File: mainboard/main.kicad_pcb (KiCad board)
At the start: 2 copper layers, 53.3 x 71.1 mm, 56 parts, among them J1 USB_OTG, J2 HIB, J3 JTAG Port, J4 C Port, J5 A Port, J6 E Port, J7 D Port, J8 B Port, J9 F Port, SW1 SW_Push, SW2 SW_Push, SW3 SW_Push, U1 LM1117-3.3, U2 TM4C123GH6PM, Y1 Crystal_GND24_Small, Y2 Crystal-32.768KHz

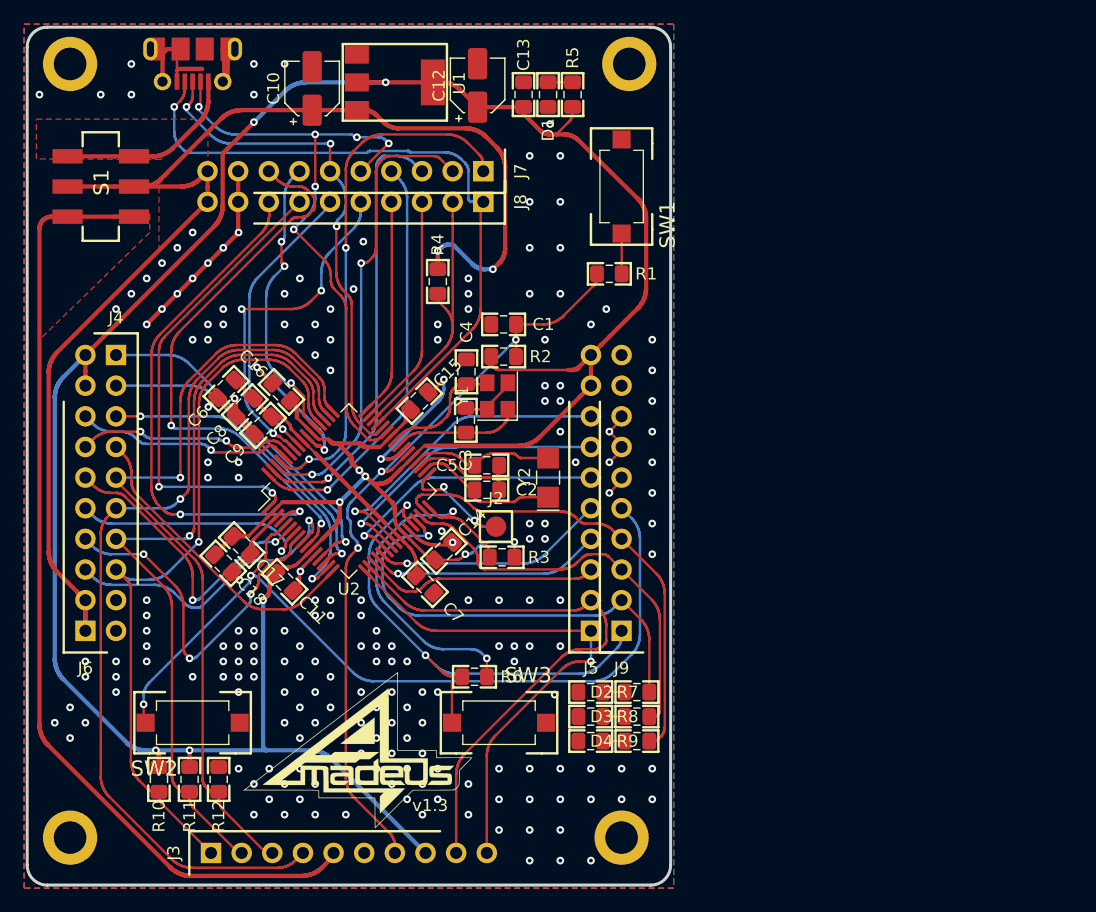
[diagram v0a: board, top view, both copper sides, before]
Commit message: Updated
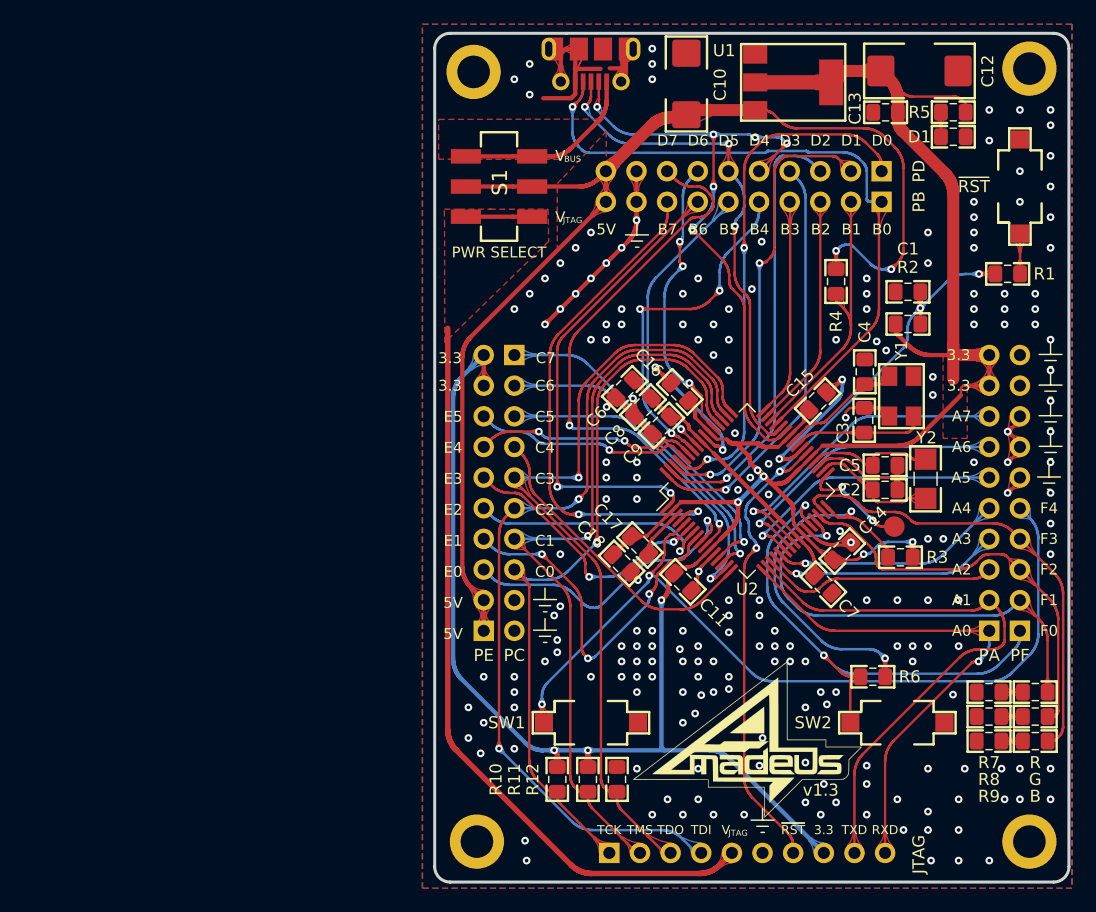
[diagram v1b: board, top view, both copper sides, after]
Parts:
- removed the G*** at (125.5, 117.9)
- removed J4: C Port, tm4c:PinHeader_1x10_P2.54mm_Vertical
- added ?: , , F.Cu at (137.9, 77.0)
- added ?: , , F.Cu at (173.1, 93.9)
- added ?: , , F.Cu at (172.2, 94.2)
- added ?: , , F.Cu at (172.8, 94.0)
- added ?: , , F.Cu at (158.1, 114.6)
- added G***: LOGO, tm4c:Steins_gate, B.Cu at (172.3, 119.4)
- added PWR SELECT: PC, tm4c:PinHeader_1x10_P2.54mm_Vertical, F.Cu at (138.4, 85.1)
- added REF**: Earth, tm4c:Earth, F.Cu at (159.0, 122.7)
- added REF**: KiCad-Logo2_8mm_SilkScreen, tm4c:KiCad-Logo2_8mm_SilkScreen, B.Cu at (150.2, 116.8)
- added REF**: Earth, tm4c:Earth, F.Cu at (141.0, 106.9)
- added REF**: Earth, tm4c:Earth, F.Cu at (141.0, 104.4)
- added REF**: Earth, tm4c:Earth, F.Cu at (148.6, 74.2)
- added REF**: Earth, tm4c:Earth, F.Cu at (182.8, 94.2)
- added REF**: Earth, tm4c:Earth, F.Cu at (182.9, 91.7)
- added REF**: Earth, tm4c:Earth, F.Cu at (182.9, 89.2)
- added REF**: Earth, tm4c:Earth, F.Cu at (182.9, 86.6)
- added REF**: Earth, tm4c:Earth, F.Cu at (182.9, 84.1)
- C10: footprint tm4c:CP_Elec_4x5.4 -> tm4c:tantalum6032
- C12: footprint tm4c:CP_Elec_4x5.4 -> tm4c:tantalum7343
- Y1: footprint Crystal:Crystal_SMD_3225-4Pin_3.2x2.5mm -> Crystal:Crystal_SMD_5032-4Pin_5.0x3.2mm
- moved C12 36.6 mm to (172.0, 61.5), turned to 0 degrees
- moved H1 33.8 mm to (181.1, 125.4)
- moved D1 33.8 mm to (174.8, 67.0), turned to 180 degrees
- moved H2 33.7 mm to (135.3, 125.4)
- moved C1 33.6 mm to (171.1, 79.8)
- moved R2 33.6 mm to (171.1, 82.5)
- moved Y1 33.5 mm to (170.5, 88.5)
- moved H4 33.5 mm to (135.1, 61.6)
- moved H3 33.2 mm to (181.1, 61.3)
- moved B 33.0 mm to (181.6, 117.1)
- moved C11 33.0 mm to (152.4, 103.9)
- moved C14 33.0 mm to (165.6, 101.3)
- moved C3 33.0 mm to (167.4, 90.5)
- moved C6 33.0 mm to (147.6, 87.9)
- moved C7 33.0 mm to (164.0, 104.1)
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- renumbered D4 to B, D3 to G, J3 to JTAG, J5 to PA, J8 to PB, J7 to PD, J6 to PE, J9 to PF, D2 to R, SW2 to SW1, SW3 to SW2, SW1 to ~RST
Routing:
- net +3V3: track 262.7 -> 230.2 mm, vias 10 -> 8
- net /VDEBUG: track 80.3 -> 68.2 mm
- net +5V: track 110.3 -> 100.6 mm
- net Earth: track 92.8 -> 100.8 mm, vias 204 -> 207
- net /GNDX: track 17.6 -> 12.8 mm
- net /PC2: track 74.1 -> 71.3 mm, vias 1 -> 2
- net /PE3: track 25.0 -> 22.3 mm
- net /PA6: track 27.0 -> 24.8 mm
- net Net-(C2-Pad1): track 12.2 -> 10.4 mm
- net /~RESET: track 64.3 -> 66.1 mm, vias 3 -> 4
- net Net-(C5-Pad2): track 11.9 -> 10.7 mm
- net /PA0: track 43.5 -> 42.7 mm
- net Net-(C3-Pad2): track 10.5 -> 11.1 mm
- net /PC5: vias 2 -> 1
- net (no net): vias 2 -> 3
- added copper zone on F.Cu, net +3V3
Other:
- board size 53.3 x 71.1 mm -> 52.6 x 70.4 mm
- board text added: "3.3"
- board text added: "5V"
- board text added: "A0"
- board text added: "A1"
- board text added: "A2"
- board text added: "A3"
- board text added: "A4"
- board text added: "A5"
- board text added: "A6"
- board text added: "A7"
- board text added: "B0"
- board text added: "B1"
- board text added: "B2"
- board text added: "B3"
- board text added: "B4"
- board text added: "B5"
- board text added: "B6"
- board text added: "B7"
- board text added: "BUS"
- board text added: "C0"
- board text added: "C1"
- board text added: "C2"
- board text added: "C3"
- board text added: "C4"
- board text added: "C5"
- board text added: "C6"
- board text added: "C7"
- board text added: "D0"
- board text added: "D1"
- board text added: "D2"
- board text added: "D3"
- board text added: "D4"
- board text added: "D5"
- board text added: "D6"
- board text added: "D7"
- board text added: "E0"
- board text added: "E1"
- board text added: "E2"
- board text added: "E3"
- board text added: "E4"
- board text added: "E5"
- board text added: "F0"
- board text added: "F1"
- board text added: "F2"
- board text added: "F3"
- board text added: "F4"
- board text added: "JTAG"
- board text added: "RXD"
- board text added: "TCK"
- board text added: "TDI"
- board text added: "TDO"
- board text added: "TMS"
- board text added: "TXD"
- board text added: "V"
- board text added: "~RST"
- board text removed: "16"
